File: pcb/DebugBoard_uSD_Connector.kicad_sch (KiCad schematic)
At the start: 6 parts, among them J4 0472192001

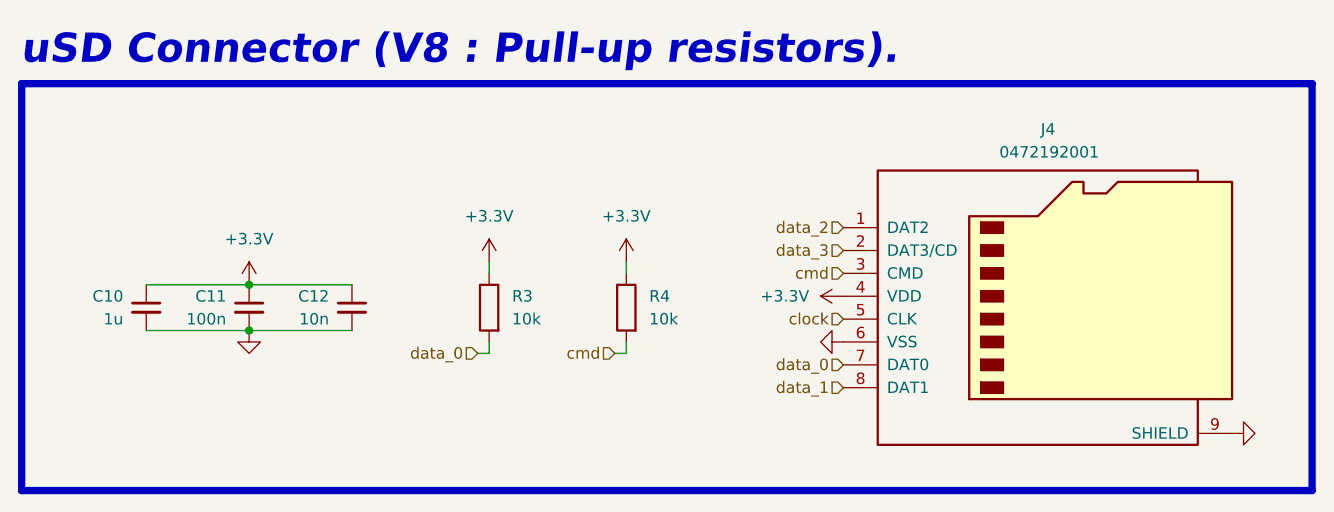
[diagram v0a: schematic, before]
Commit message: Laid out and routed `DebugBoard`.
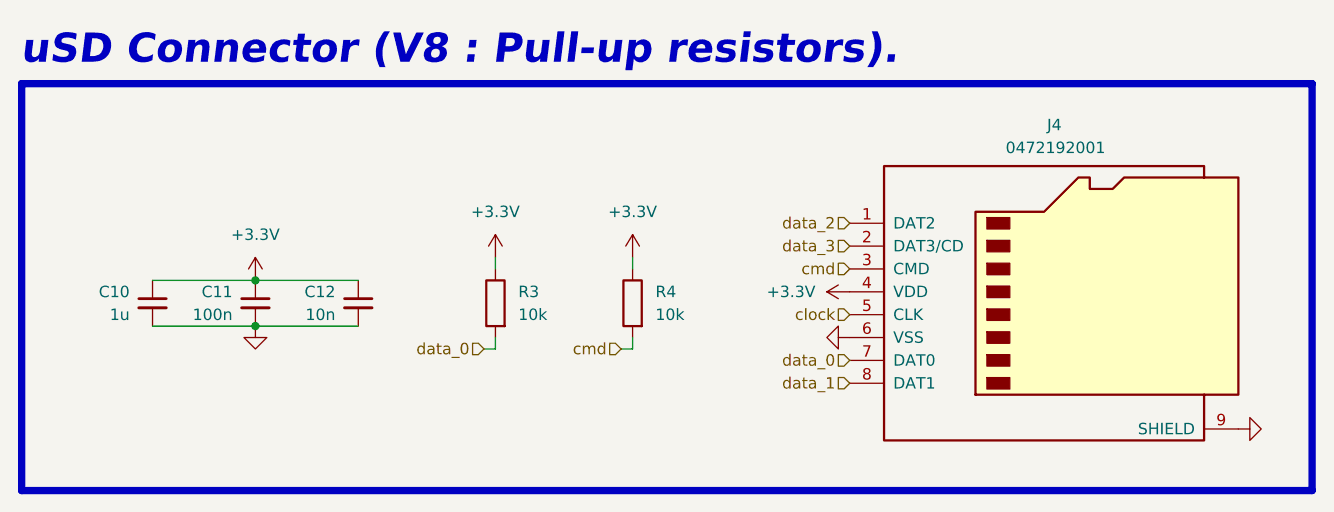
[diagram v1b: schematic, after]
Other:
- moved on the sheet: C10, C11, C12, J4, R3, R4
